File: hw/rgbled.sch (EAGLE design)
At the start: 1 part, among them U1 ATTINY85-20P

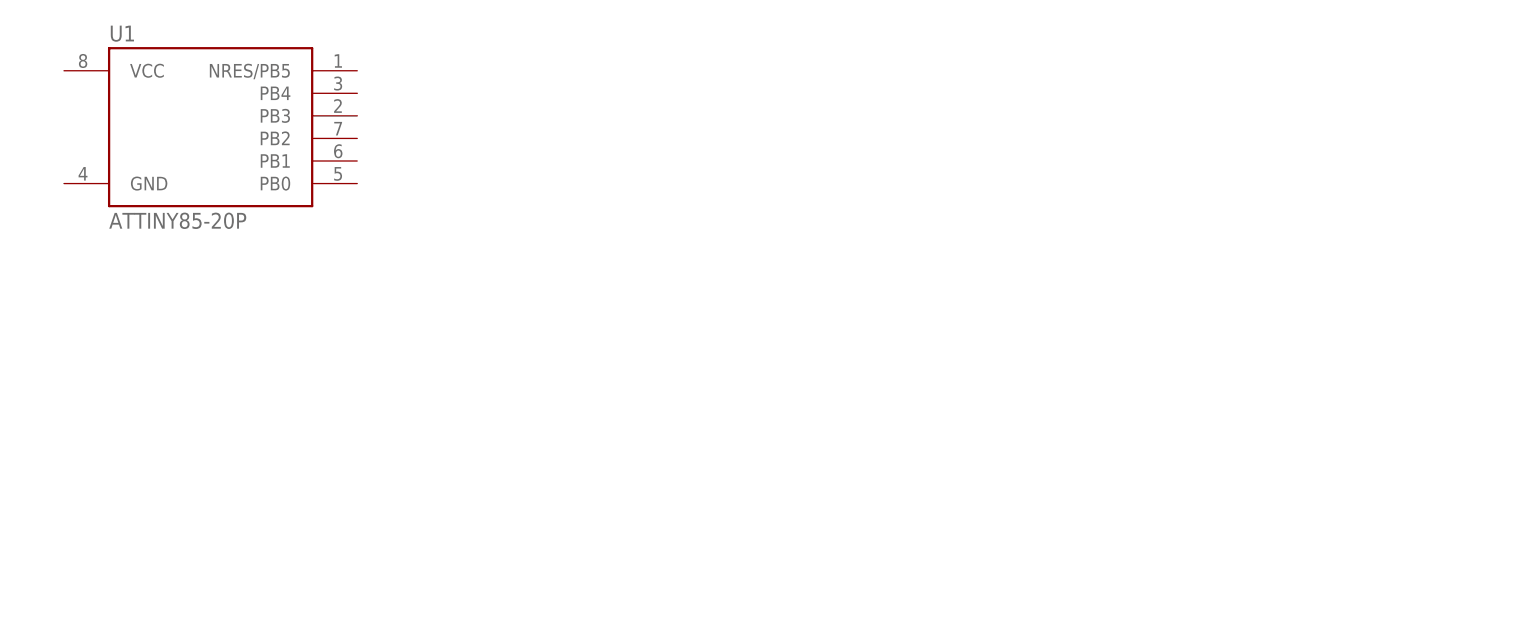
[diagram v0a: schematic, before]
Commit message: v1 boardu
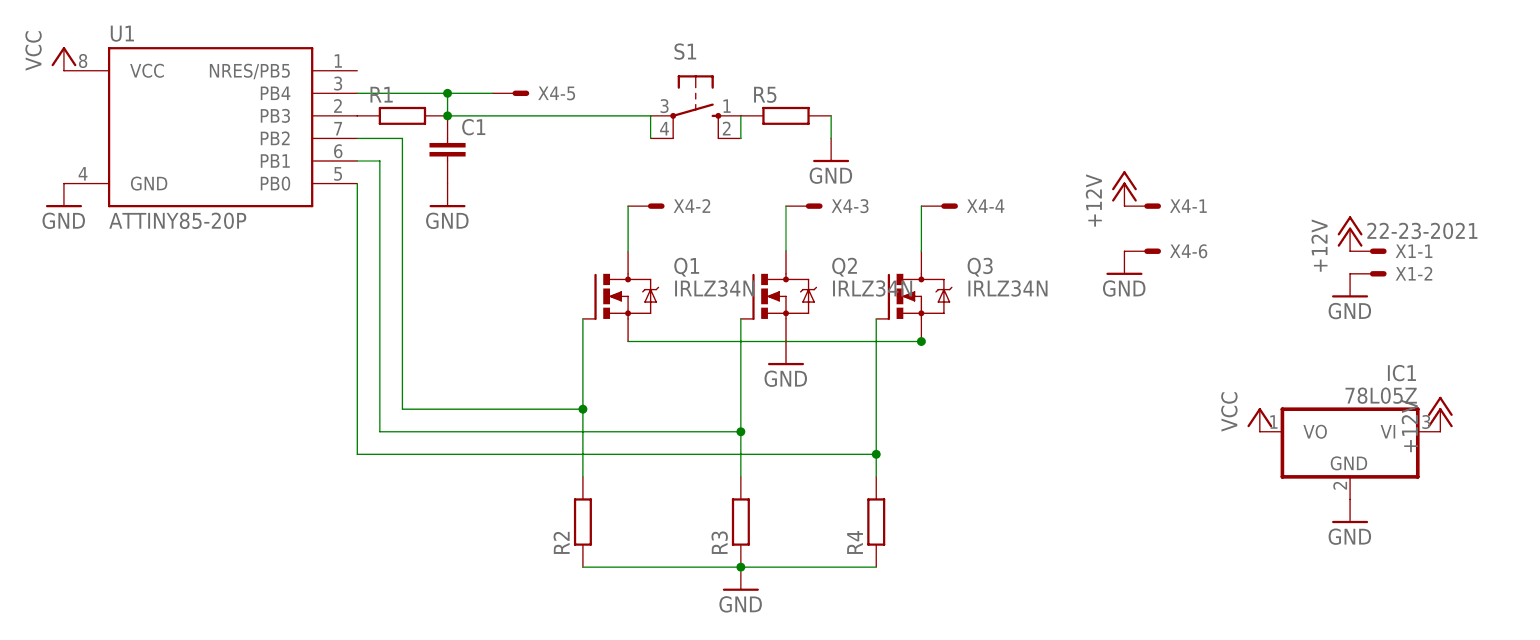
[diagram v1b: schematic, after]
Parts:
- added C1: (no value), resistor:C-EU025-024X044
- added IC1: 78L05Z, linear:78L05Z
- added Q1, Q2, Q3: IRLZ34N, transistor-power:IRF540
- added R1, R2, R3, R4, R5: (no value), resistor:R-EU_0204/5
- added S1: (no value), switch-omron:10-XX
- added X1: 22-23-2021, con-molex:22-23-2021
- added X4: (no value), con-molex:22-23-2061
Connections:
- new net +12V: IC1.VI, X1-1.S, X4-1.S
- new net GND: C1.2, IC1.GND, Q1.S, Q2.S, Q3.S, R2.1, R3.1, R4.1, R5.2, U1.GND, X1-2.S, X4-6.S
- new net N$1: R5.1, S1.S, S1.S1
- new net N$10: Q3.G, R4.2, U1.PB0
- new net N$11: Q2.G, R3.2, U1.PB1
- new net N$12: Q1.G, R2.2, U1.PB2
- new net N$2: Q1.D, X4-2.S
- new net N$3: Q2.D, X4-3.S
- new net N$4: Q3.D, X4-4.S
- new net N$5: R1.1, U1.PB3
- new net N$7: C1.1, R1.2, S1.P, S1.P1, U1.PB4, X4-5.S
- new net VCC: IC1.VO, U1.VCC
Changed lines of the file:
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@@
 <parts>
 <part name="U1" library="_hhn_attiny25_45_85" deviceset="ATTINY85*" device="P" technology="-20"/>
+<part name="Q1" library="transistor-power" deviceset="IRF540" device="" value="IRLZ34N"/>
+<part name="Q2" library="transistor-power" deviceset="IRF540" device="" value="IRLZ34N"/>
+<part name="Q3" library="transistor-power" deviceset="IRF540" device="" value="IRLZ34N"/>
+<part name="X1" library="con-molex" deviceset="22-23-2021" device=""/>
+<part name="X4" library="con-molex" deviceset="22-23-2061" device=""/>
+<part name="GND1" library="supply1" deviceset="GND" device=""/>
+<part name="GND2" library="supply1" deviceset="GND" device=""/>
+<part name="P+1" library="supply1" deviceset="+12V" device=""/>
+<part name="P+2" library="supply1" deviceset="VCC" device=""/>
+<part name="P+3" library="supply1" deviceset="+12V" device=""/>
+<part name="GND3" library="supply1" deviceset="GND" device=""/>
+<part name="P+4" library="supply1" deviceset="VCC" device=""/>
+<part name="IC1" library="linear" deviceset="78*" device="Z" technology="L05"/>
+<part name="GND4" library="supply1" deviceset="GND" device=""/>
+<part name="P+5" library="supply1" deviceset="+12V" device=""/>
+<part name="GND5" library="supply1" deviceset="GND" device=""/>
+<part name="R1" library="resistor" deviceset="R-EU_" device="0204/5"/>
+<part name="C1" library="resistor" deviceset="C-EU" device="025-024X044"/>
+<part name="GND6" library="supply1" deviceset="GND" device=""/>
+<part name="R2" library="resistor" deviceset="R-EU_" device="0204/5"/>
+<part name="R3" library="resistor" deviceset="R-EU_" device="0204/5"/>
+<part name="R4" library="resistor" deviceset="R-EU_" device="0204/5"/>
+<part name="GND7" library="supply1" deviceset="GND" device=""/>
+<part name="S1" library="switch-omron" deviceset="10-XX" device=""/>
+<part name="GND8" library="supply1" deviceset="GND" device=""/>
+<part name="R5" library="resistor" deviceset="R-EU_" device="0204/5"/>
 </parts>
 <sheets>
@@
 <instances>
 <instance part="U1" gate="G$1" x="22.86" y="58.42"/>
+<instance part="Q1" gate="G$1" x="68.58" y="38.1"/>
+<instance part="Q2" gate="G$1" x="86.36" y="38.1"/>
+<instance part="Q3" gate="G$1" x="101.6" y="38.1"/>
+<instance part="X1" gate="-1" x="154.94" y="43.18"/>
+<instance part="X1" gate="-2" x="154.94" y="40.64"/>
+<instance part="X4" gate="-1" x="129.54" y="48.26"/>
+<instance part="X4" gate="-2" x="73.66" y="48.26"/>
+<instance part="X4" gate="-3" x="91.44" y="48.26"/>
+<instance part="X4" gate="-4" x="106.68" y="48.26"/>
+<instance part="X4" gate="-5" x="58.42" y="60.96"/>
+<instance part="X4" gate="-6" x="129.54" y="43.18"/>
+<instance part="GND1" gate="1" x="152.4" y="38.1"/>
+<instance part="GND2" gate="1" x="7.62" y="48.26"/>
+<instance part="P+1" gate="1" x="152.4" y="45.72"/>
+<instance part="P+2" gate="VCC" x="142.24" y="25.4"/>
+<instance part="P+3" gate="1" x="162.56" y="25.4"/>
+<instance part="GND3" gate="1" x="152.4" y="12.7"/>
+<instance part="P+4" gate="VCC" x="7.62" y="66.04"/>
+<instance part="IC1" gate="A1" x="152.4" y="22.86" rot="MR0"/>
+<instance part="GND4" gate="1" x="88.9" y="30.48"/>
+<instance part="P+5" gate="1" x="127" y="50.8"/>
+<instance part="GND5" gate="1" x="127" y="40.64"/>
+<instance part="R1" gate="G$1" x="45.72" y="58.42"/>
+<instance part="C1" gate="G$1" x="50.8" y="55.88"/>
+<instance part="GND6" gate="1" x="50.8" y="48.26"/>
+<instance part="R2" gate="G$1" x="66.04" y="12.7" rot="R90"/>
+<instance part="R3" gate="G$1" x="83.82" y="12.7" rot="R90"/>
+<instance part="R4" gate="G$1" x="99.06" y="12.7" rot="R90"/>
+<instance part="GND7" gate="1" x="83.82" y="5.08"/>
+<instance part="S1" gate="1" x="78.74" y="58.42" rot="R270"/>
+<instance part="GND8" gate="1" x="93.98" y="53.34"/>
+<instance part="R5" gate="G$1" x="88.9" y="58.42"/>
 </instances>
 <busses>
 </busses>
 <nets>
+<net name="GND" class="0">
+<segment>
+<pinref part="X1" gate="-2" pin="S"/>
+<pinref part="GND1" gate="1" pin="GND"/>
+</segment>
+<segment>
+<pinref part="U1" gate="G$1" pin="GND"/>
+<pinref part="GND2" gate="1" pin="GND"/>
+</segment>
+<segment>
+<pinref part="IC1" gate="A1" pin="GND"/>
+<pinref part="GND3" gate="1" pin="GND"/>
+</segment>
+<segment>
+<pinref part="Q1" gate="G$1" pin="S"/>
+<pinref part="Q2" gate="G$1" pin="S"/>
+<wire x1="71.12" y1="33.02" x2="88.9" y2="33.02" width="0.1524" layer="91"/>
+<pinref part="Q3" gate="G$1" pin="S"/>
+<pinref part="GND4" gate="1" pin="GND"/>
+<wire x1="104.14" y1="33.02" x2="88.9" y2="33.02" width="0.1524" layer="91"/>
+<junction x="104.14" y="33.02"/>
+</segment>
+<segment>
+<pinref part="X4" gate="-6" pin="S"/>
+<pinref part="GND5" gate="1" pin="GND"/>
+</segment>
+<segment>
+<pinref part="C1" gate="G$1" pin="2"/>
+<pinref part="GND6" gate="1" pin="GND"/>
+</segment>
+<segment>
+<pinref part="R2" gate="G$1" pin="1"/>
+<pinref part="R3" gate="G$1" pin="1"/>
+<wire x1="66.04" y1="7.62" x2="83.82" y2="7.62" width="0.1524" layer="91"/>
+<pinref part="R4" gate="G$1" pin="1"/>
+<wire x1="83.82" y1="7.62" x2="99.06" y2="7.62" width="0.1524" layer="91"/>
+<pinref part="GND7" gate="1" pin="GND"/>
+<junction x="83.82" y="7.62"/>
+</segment>
+<segment>
+<pinref part="R5" gate="G$1" pin="2"/>
+<pinref part="GND8" gate="1" pin="GND"/>
+<wire x1="93.98" y1="58.42" x2="93.98" y2="55.88" width="0.1524" layer="91"/>
+</segment>
+</net>
+<net name="+12V" class="0">
+<segment>
+<pinref part="X1" gate="-1" pin="S"/>
+<pinref part="P+1" gate="1" pin="+12V"/>
+</segment>
+<segment>
+<pinref part="IC1" gate="A1" pin="VI"/>
+<pinref part="P+3" gate="1" pin="+12V"/>
+</segment>
+<segment>
+<pinref part="X4" gate="-1" pin="S"/>
+<pinref part="P+5" gate="1" pin="+12V"/>
+</segment>
+</net>
+<net name="VCC" class="0">
+<segment>
+<pinref part="IC1" gate="A1" pin="VO"/>
+<pinref part="P+2" gate="VCC" pin="VCC"/>
+</segment>
+<segment>
+<pinref part="U1" gate="G$1" pin="VCC"/>
+<pinref part="P+4" gate="VCC" pin="VCC"/>
+</segment>
+</net>
+<net name="N$2" class="0">
+<segment>
+<pinref part="X4" gate="-2" pin="S"/>
+<pinref part="Q1" gate="G$1" pin="D"/>
+<wire x1="71.12" y1="48.26" x2="71.12" y2="43.18" width="0.1524" layer="91"/>
+</segment>
+</net>
+<net name="N$3" class="0">
+<segment>
+<pinref part="X4" gate="-3" pin="S"/>
+<pinref part="Q2" gate="G$1" pin="D"/>
+<wire x1="88.9" y1="48.26" x2="88.9" y2="43.18" width="0.1524" layer="91"/>
+</segment>
+</net>
+<net name="N$4" class="0">
+<segment>
+<pinref part="X4" gate="-4" pin="S"/>
+<pinref part="Q3" gate="G$1" pin="D"/>
+<wire x1="104.14" y1="48.26" x2="104.14" y2="43.18" width="0.1524" layer="91"/>
+</segment>
+</net>
+<net name="N$5" class="0">
+<segment>
+<pinref part="U1" gate="G$1" pin="PB3"/>
+<pinref part="R1" gate="G$1" pin="1"/>
+</segment>
+</net>
+<net name="N$10" class="0">
+<segment>
+<pinref part="Q3" gate="G$1" pin="G"/>
+<wire x1="99.06" y1="35.56" x2="99.06" y2="20.32" width="0.1524" layer="91"/>
+<pinref part="R4" gate="G$1" pin="2"/>
+<pinref part="U1" gate="G$1" pin="PB0"/>
+<wire x1="99.06" y1="20.32" x2="99.06" y2="17.78" width="0.1524" layer="91"/>
+<wire x1="99.06" y1="20.32" x2="40.64" y2="20.32" width="0.1524" layer="91"/>
+<wire x1="40.64" y1="20.32" x2="40.64" y2="50.8" width="0.1524" layer="91"/>
+<junction x="99.06" y="20.32"/>
+</segment>
+</net>
+<net name="N$11" class="0">
+<segment>
+<pinref part="Q2" gate="G$1" pin="G"/>
+<wire x1="83.82" y1="35.56" x2="83.82" y2="22.86" width="0.1524" layer="91"/>
+<pinref part="R3" gate="G$1" pin="2"/>
+<wire x1="83.82" y1="22.86" x2="83.82" y2="17.78" width="0.1524" layer="91"/>
+<wire x1="83.82" y1="22.86" x2="43.18" y2="22.86" width="0.1524" layer="91"/>
+<wire x1="43.18" y1="22.86" x2="43.18" y2="53.34" width="0.1524" layer="91"/>
+<pinref part="U1" gate="G$1" pin="PB1"/>
+<wire x1="43.18" y1="53.34" x2="40.64" y2="53.34" width="0.1524" layer="91"/>
+<junction x="83.82" y="22.86"/>
+</segment>
+</net>
+<net name="N$12" class="0">
+<segment>
+<pinref part="Q1" gate="G$1" pin="G"/>
+<wire x1="66.04" y1="35.56" x2="66.04" y2="25.4" width="0.1524" layer="91"/>
+<pinref part="R2" gate="G$1" pin="2"/>
+<wire x1="66.04" y1="25.4" x2="66.04" y2="17.78" width="0.1524" layer="91"/>
+<wire x1="66.04" y1="25.4" x2="45.72" y2="25.4" width="0.1524" layer="91"/>
+<wire x1="45.72" y1="25.4" x2="45.72" y2="55.88" width="0.1524" layer="91"/>
+<pinref part="U1" gate="G$1" pin="PB2"/>
+<wire x1="45.72" y1="55.88" x2="40.64" y2="55.88" width="0.1524" layer="91"/>
+<junction x="66.04" y="25.4"/>
+</segment>
+</net>
+<net name="N$7" class="0">
+<segment>
+<pinref part="R1" gate="G$1" pin="2"/>
+<pinref part="C1" gate="G$1" pin="1"/>
+<pinref part="X4" gate="-5" pin="S"/>
+<pinref part="U1" gate="G$1" pin="PB4"/>
+<wire x1="40.64" y1="60.96" x2="50.8" y2="60.96" width="0.1524" layer="91"/>
+<wire x1="50.8" y1="60.96" x2="55.88" y2="60.96" width="0.1524" layer="91"/>
+<wire x1="50.8" y1="60.96" x2="50.8" y2="58.42" width="0.1524" layer="91"/>
+<pinref part="S1" gate="1" pin="P"/>
+<wire x1="50.8" y1="58.42" x2="73.66" y2="58.42" width="0.1524" layer="91"/>
+<pinref part="S1" gate="1" pin="P1"/>
+<wire x1="73.66" y1="58.42" x2="73.66" y2="55.88" width="0.1524" layer="91"/>
+<junction x="50.8" y="60.96"/>
+<junction x="50.8" y="58.42"/>
+</segment>
+</net>
+<net name="N$1" class="0">
+<segment>
+<pinref part="S1" gate="1" pin="S"/>
+<pinref part="R5" gate="G$1" pin="1"/>
+<pinref part="S1" gate="1" pin="S1"/>
+<wire x1="83.82" y1="58.42" x2="83.82" y2="55.88" width="0.1524" layer="91"/>
+</segment>
+</net>
 </nets>
 </sheet>
